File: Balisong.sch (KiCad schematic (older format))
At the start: 14 parts

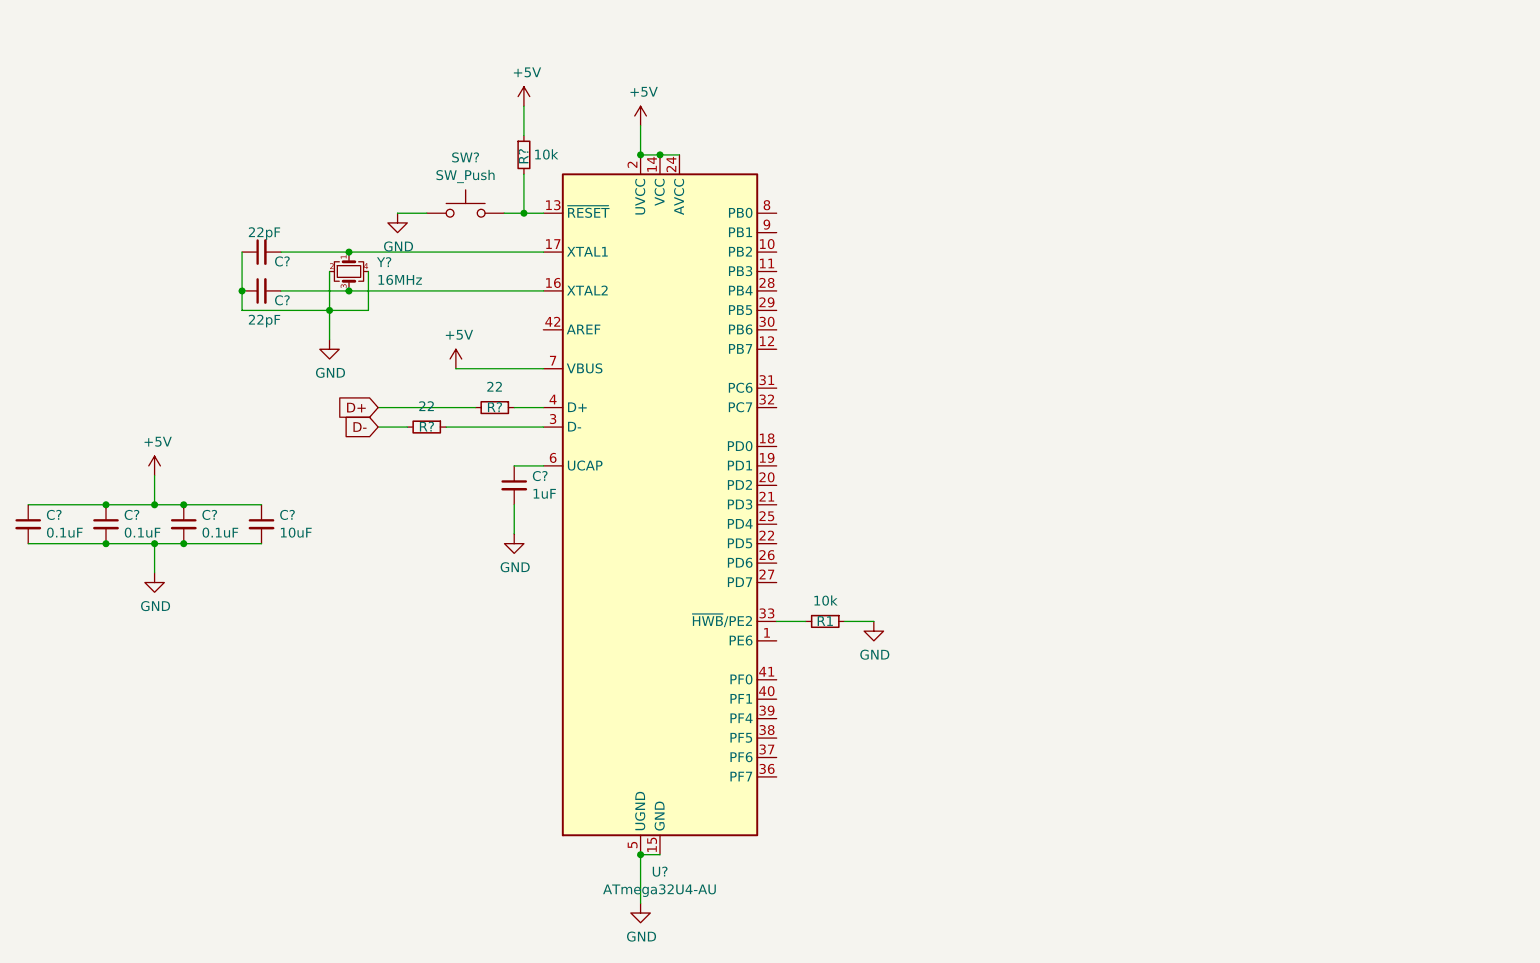
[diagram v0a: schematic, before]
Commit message: The rest of the schematic
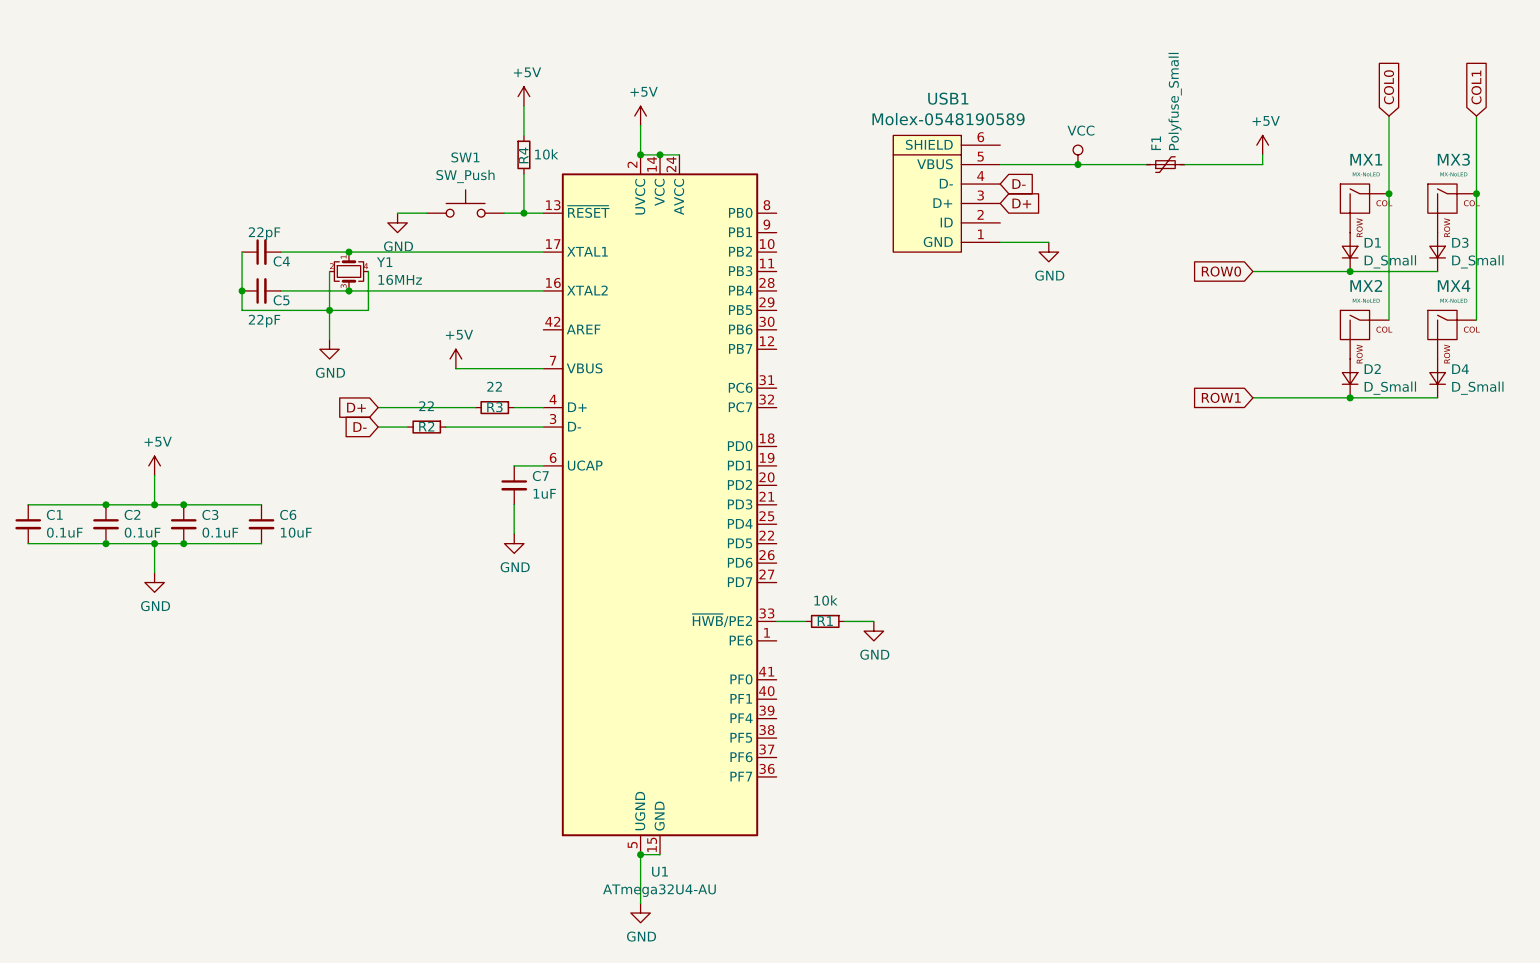
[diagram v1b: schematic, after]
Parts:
- added D1, D2, D3, D4: D_Small, Diode_SMD:D_SOD-123, symbol Device:D_Small
- added F1: Polyfuse_Small, Fuse:Fuse_1206_3216Metric_Pad1.42x1.75mm_HandSolder, symbol Device:Polyfuse_Small
- added MX1, MX2, MX3, MX4: MX-NoLED, MX_Alps_Hybrid:MX-1U-NoLED, symbol MX_Alps_Hybrid:MX-NoLED
- added USB1: Molex-0548190589, random-keyboard-parts:Molex-0548190589, symbol random-keyboard-parts:Molex-0548190589
- C1, C2, C3, C4, C5, C6, C7: renamed from C?; footprint (none) -> Capacitor_SMD:C_0805_2012Metric
- R1: footprint (none) -> Resistor_SMD:R_0805_2012Metric
- R2, R3, R4: renamed from R?; footprint (none) -> Resistor_SMD:R_0805_2012Metric
- SW1: renamed from SW?; footprint (none) -> random-keyboard-parts:SKQG-1155865
- Y1: renamed from Y?; footprint (none) -> Crystal:Crystal_SMD_3225-4Pin_3.2x2.5mm
- gave numbers to parts that had none: 1
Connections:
- net +5V: now also F1.2
- net D+: now also USB1.3 (D+)
- net D-: now also USB1.4 (D-)
- net GND: now also USB1.1 (GND)
- new net: D3.2 (A), MX3.2 (ROW)
- new net: D1.2 (A), MX1.2 (ROW)
- new net: D2.2 (A), MX2.2 (ROW)
- new net: D4.2 (A), MX4.2 (ROW)
- new net COL0: MX1.1 (COL), MX2.1 (COL)
- new net COL1: MX3.1 (COL), MX4.1 (COL)
- new net ROW0: D1.1 (K), D3.1 (K)
- new net ROW1: D2.1 (K), D4.1 (K)
- new net VCC: F1.1, USB1.5 (VBUS)
